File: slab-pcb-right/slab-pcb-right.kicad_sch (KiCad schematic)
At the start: 126 parts, among them J1 MagnetR, J2 MagnetL, J3 TRRS_R, J4 TRRS_L, J5 SSD1306, J6 Conn_01x06, SW1 RotaryEncoder, U1 Seeeduino Xiao rp2040, U2 PCA9555PW, U3 PCA9555PW, U4 ADS1110, U5 SN74AHCT125PWR

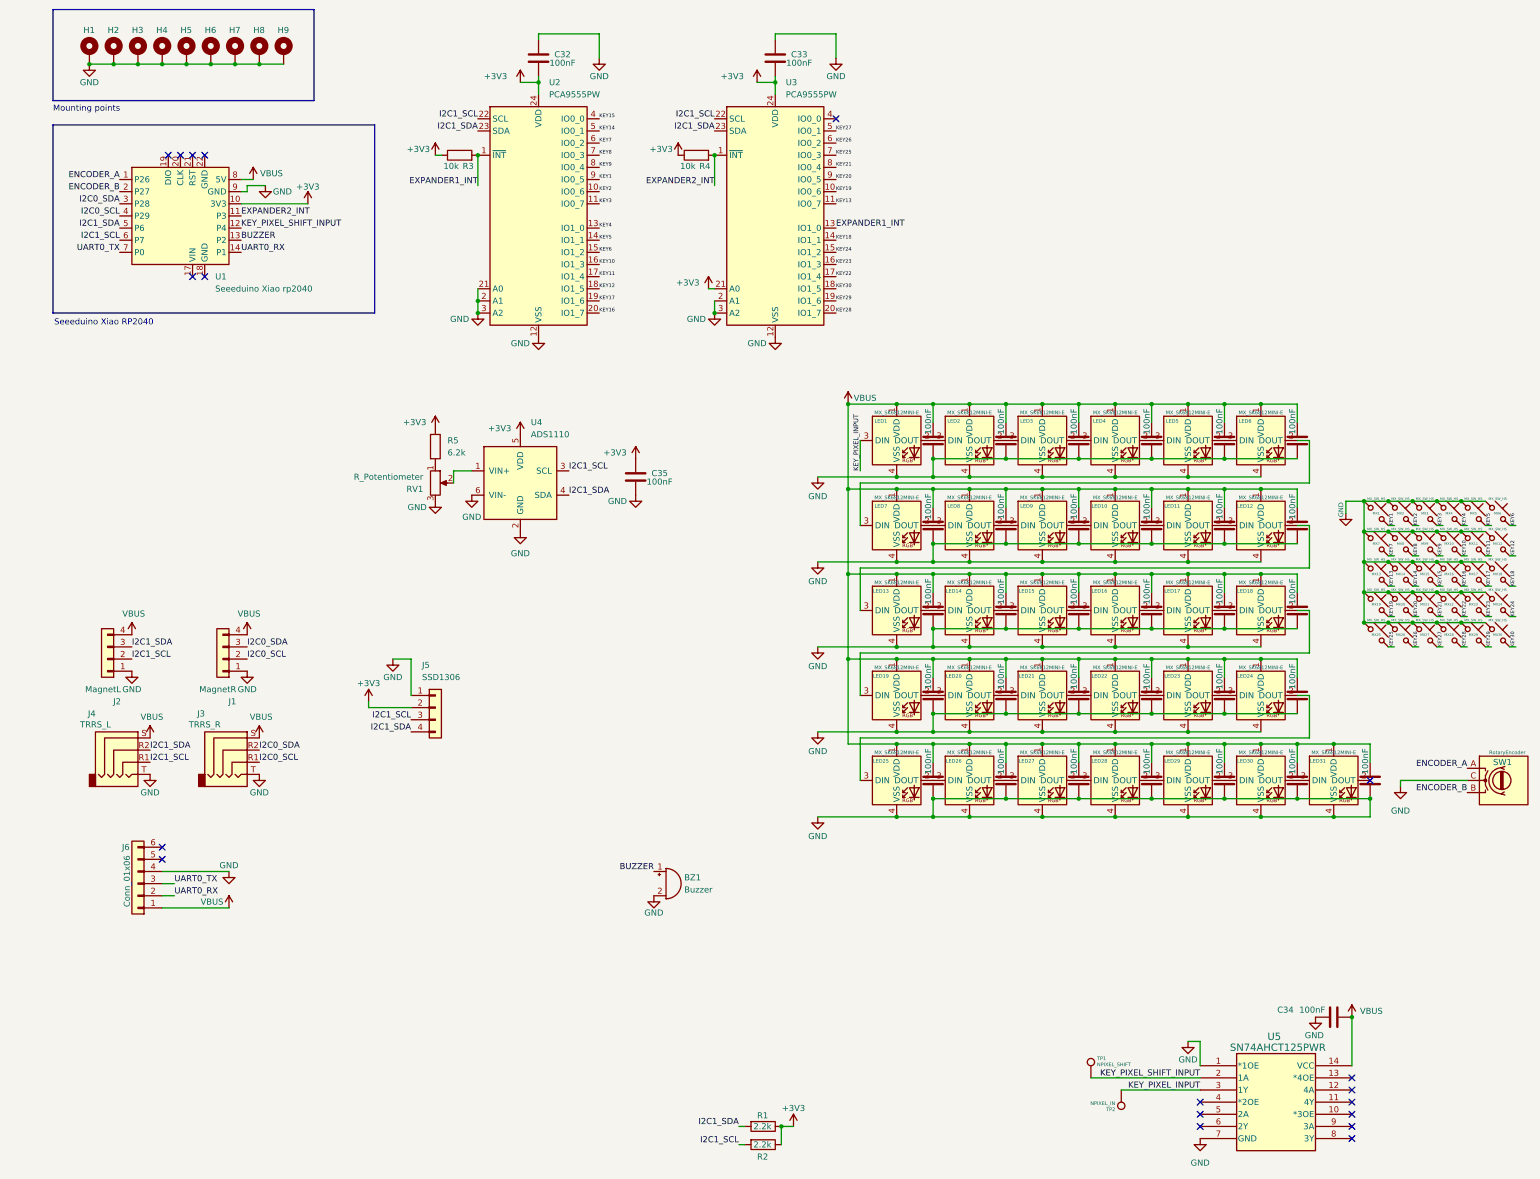
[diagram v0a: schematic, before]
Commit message: feat: start on v4, updated: right-hand schematic
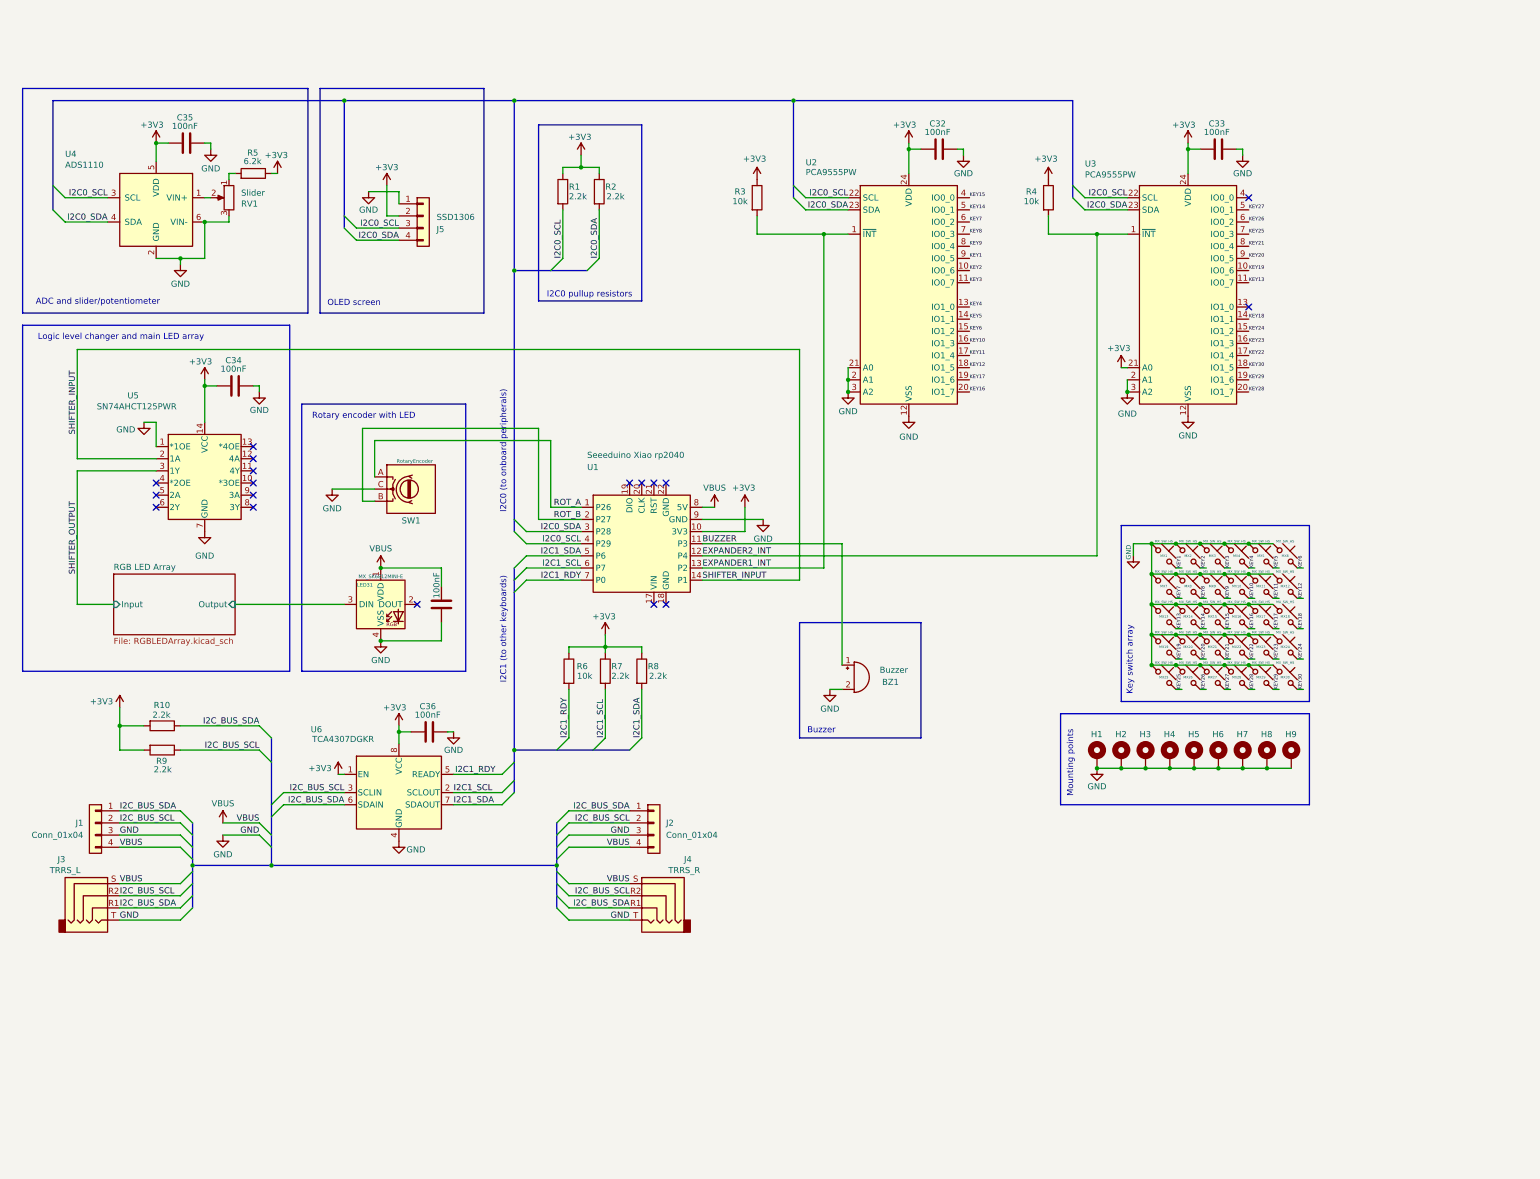
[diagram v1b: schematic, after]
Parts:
- removed C1, C10, C11, C12, C13, C14, C15, C16, C17, C18, C19, C2, C20, C21, C22, C23, C24, C25, C26, C27, C28, C29, C3, C30, C4, C5, C6, C7, C8, C9: 100nF, Capacitor_SMD:C_0603_1608Metric_Pad1.08x0.95mm_HandSolder, symbol Device:C
- removed J6: Conn_01x06, Connector_PinHeader_2.54mm:PinHeader_1x06_P2.54mm_Vertical, symbol Connector_Generic:Conn_01x06
- removed LED1, LED10, LED11, LED12, LED13, LED14, LED15, LED16, LED17, LED18, LED19, LED2, LED20, LED21, LED22, LED23, LED24, LED25, LED26, LED27, LED28, LED29, LED3, LED30, LED4, LED5, LED6, LED7, LED8, LED9: MX_SK6812MINI-E, CustomFootprints:LED_MX_6028R-ROT_Custom, symbol PCM_marbastlib-mx:MX_SK6812MINI-E
- removed TP1: NPIXEL_SHIFT, TestPoint:TestPoint_Pad_1.0x1.0mm, symbol Connector:TestPoint
- removed TP2: NPIXEL_IN, TestPoint:TestPoint_Pad_1.0x1.0mm, symbol Connector:TestPoint
- added C36: 100nF, Capacitor_SMD:C_0603_1608Metric_Pad1.08x0.95mm_HandSolder, symbol Device:C
- added R10, R7, R8, R9: 2.2k, Resistor_SMD:R_0603_1608Metric_Pad0.98x0.95mm_HandSolder, symbol Device:R
- added R6: 10k, Resistor_SMD:R_0603_1608Metric_Pad0.98x0.95mm_HandSolder, symbol Device:R
- added U6: TCA4307DGKR, SOIC8_DGK_TEX, symbol CustomSymbols:TCA4307DGKR
- J1: value MagnetR -> Conn_01x04; footprint CustomFootprints:5358_mag_connector_1x4_pads -> (none)
- J2: value MagnetL -> Conn_01x04; footprint CustomFootprints:5358_mag_connector_1x4_pins -> (none)
- RV1: value R_Potentiometer -> Slider
- renumbered J4 to J3, J3 to J4
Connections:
- net UART0_RX is gone; now on net SHIFTER_INPUT: U1.14 (P1)
- net +3V3: now also C32.2, C33.2, C34.2, U5.14 (VCC), C36.2, R10.2, R6.1, R7.1, R8.1, R9.2, U6.1 (EN), U6.8 (VCC); no longer C32.1, C33.1
- net BUZZER: now also U1.11 (P3); no longer U1.13 (P2)
- net EXPANDER1_INT: now also U1.13 (P2); no longer U3.13 (IO1_0)
- net EXPANDER2_INT: now also U1.12 (P4); no longer U1.11 (P3)
- net GND: now also C32.1, C33.1, J1.3 (Pin_3), J2.3 (Pin_3), C36.1, U6.4 (GND); no longer C32.2, C33.2, J1.1 (Pin_1), J2.1 (Pin_1)
- net I2C0_SCL: now also J5.3 (Pin_3), R1.2, U2.22 (SCL), U3.22 (SCL), U4.3 (SCL); no longer J1.2 (Pin_2), J4.R1
- net I2C0_SDA: now also J5.4 (Pin_4), R2.2, U2.23 (SDA), U3.23 (SDA), U4.4 (SDA); no longer J1.3 (Pin_3), J4.R2
- net I2C1_SCL: now also R7.2, U6.2 (SCLOUT); no longer J2.2 (Pin_2), J3.R1, J5.3 (Pin_3), R2.2, U2.22 (SCL), U3.22 (SCL), U4.3 (SCL)
- net I2C1_SDA: now also R8.2, U6.7 (SDAOUT); no longer J2.3 (Pin_3), J3.R2, J5.4 (Pin_4), R1.2, U2.23 (SDA), U3.23 (SDA), U4.4 (SDA)
- net VBUS: no longer C34.2, U5.14 (VCC)
- net RGB LED Array/Output: now reaches LED31.3 (DIN)
- net ENCODER_A renamed ROT_A
- net ENCODER_B renamed ROT_B
- net KEY_PIXEL_INPUT renamed SHIFTER_OUTPUT
- net KEY_PIXEL_SHIFT_INPUT renamed SHIFTER_INPUT
- net SHIFTER_INPUT: no longer U1.12 (P4)
- net UART0_TX renamed I2C1_RDY
- net I2C1_RDY: now also R6.2, U6.5 (READY)
- new net I2C_BUS_SCL: J1.2 (Pin_2), J2.2 (Pin_2), J3.R2, J4.R2, R9.1, U6.3 (SCLIN)
- new net I2C_BUS_SDA: J1.1 (Pin_1), J2.1 (Pin_1), J3.R1, J4.R1, R10.1, U6.6 (SDAIN)
- no-connect marks 19 -> 18
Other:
- added sheet RGB LED Array (RGBLEDArray.kicad_sch)
- note added: "ADC and slider/potentiometer"
- note added: "Buzzer"
- note added: "I2C0 (to onboard peripherals)"
- note added: "I2C0 pullup resistors"
- note added: "I2C1 (to other keyboards)"
- note added: "Key switch array"
- note added: "Logic level changer and main LED array"
- note added: "OLED screen"
- note added: "Rotary encoder with LED"
- note removed: "Seeeduino Xiao RP2040"
- title: The Slab Keyboard - Right Module -> The Interchange Keyboard - Right Module
- moved on the sheet: BZ1, C32, H1, H2, H3, H4, H5, H6, H7, H8, H9, J3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
